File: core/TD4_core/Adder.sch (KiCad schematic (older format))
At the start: 30 parts

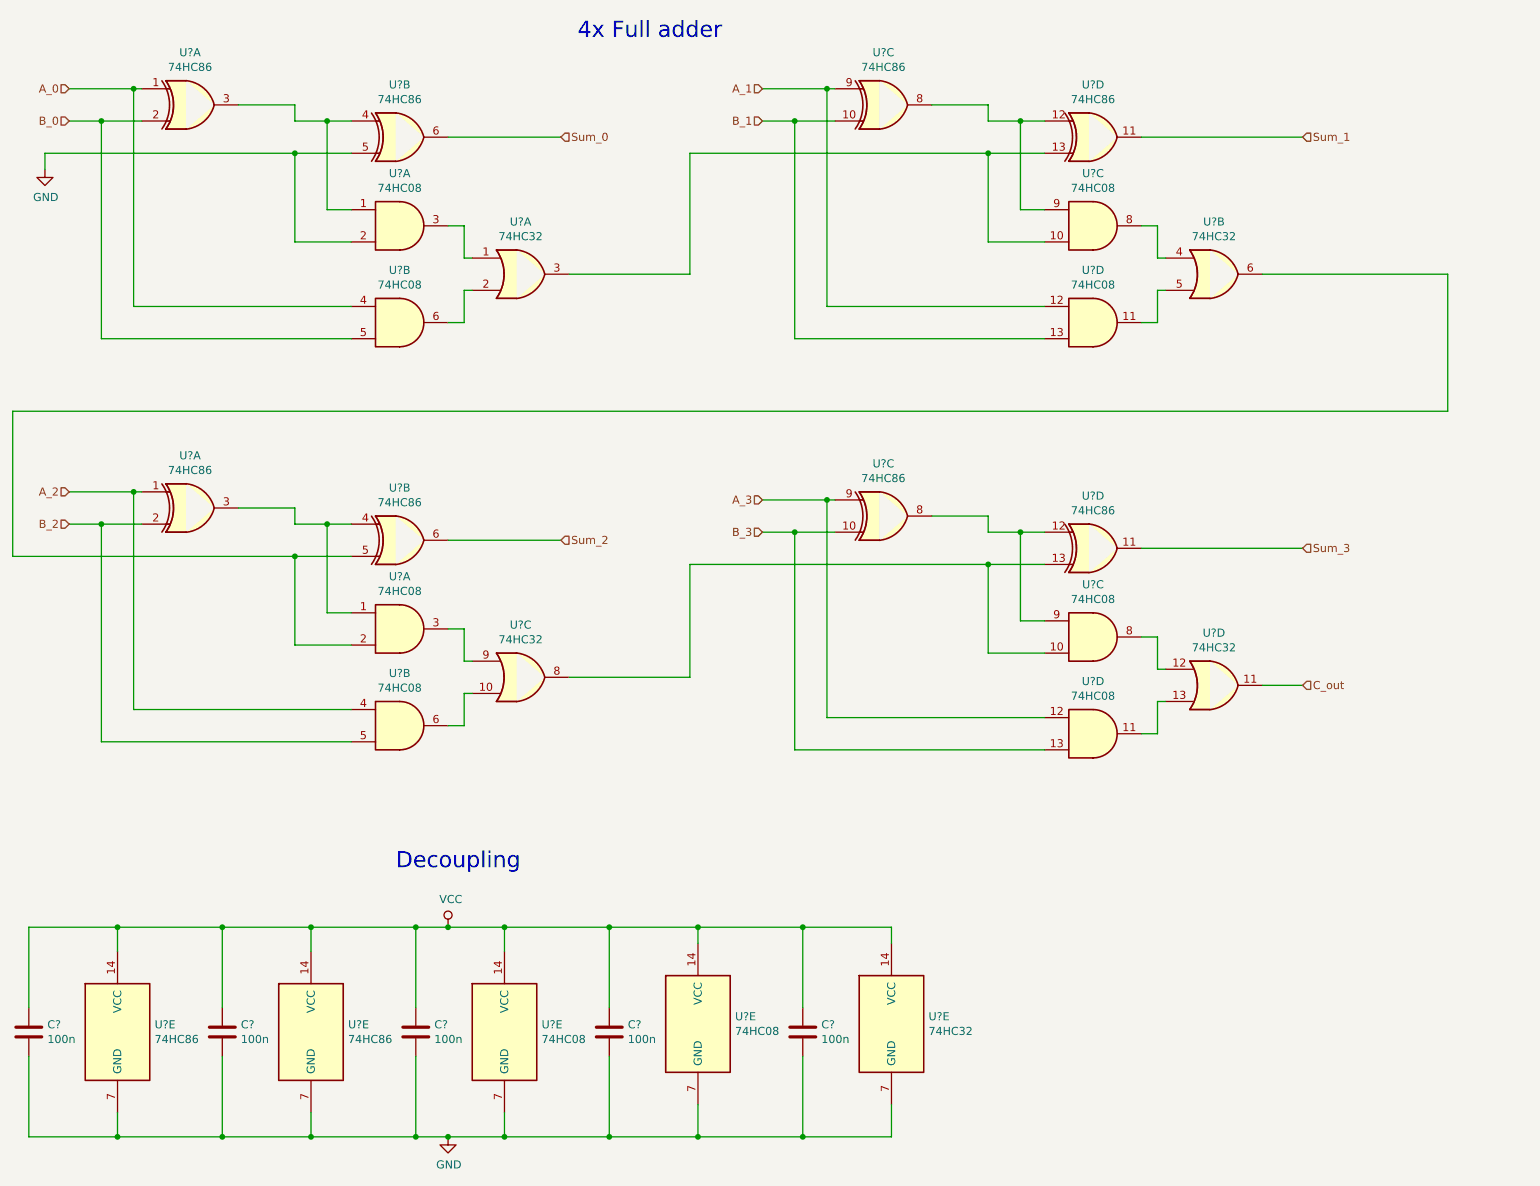
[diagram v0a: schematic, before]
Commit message: RAM refactoring goes on
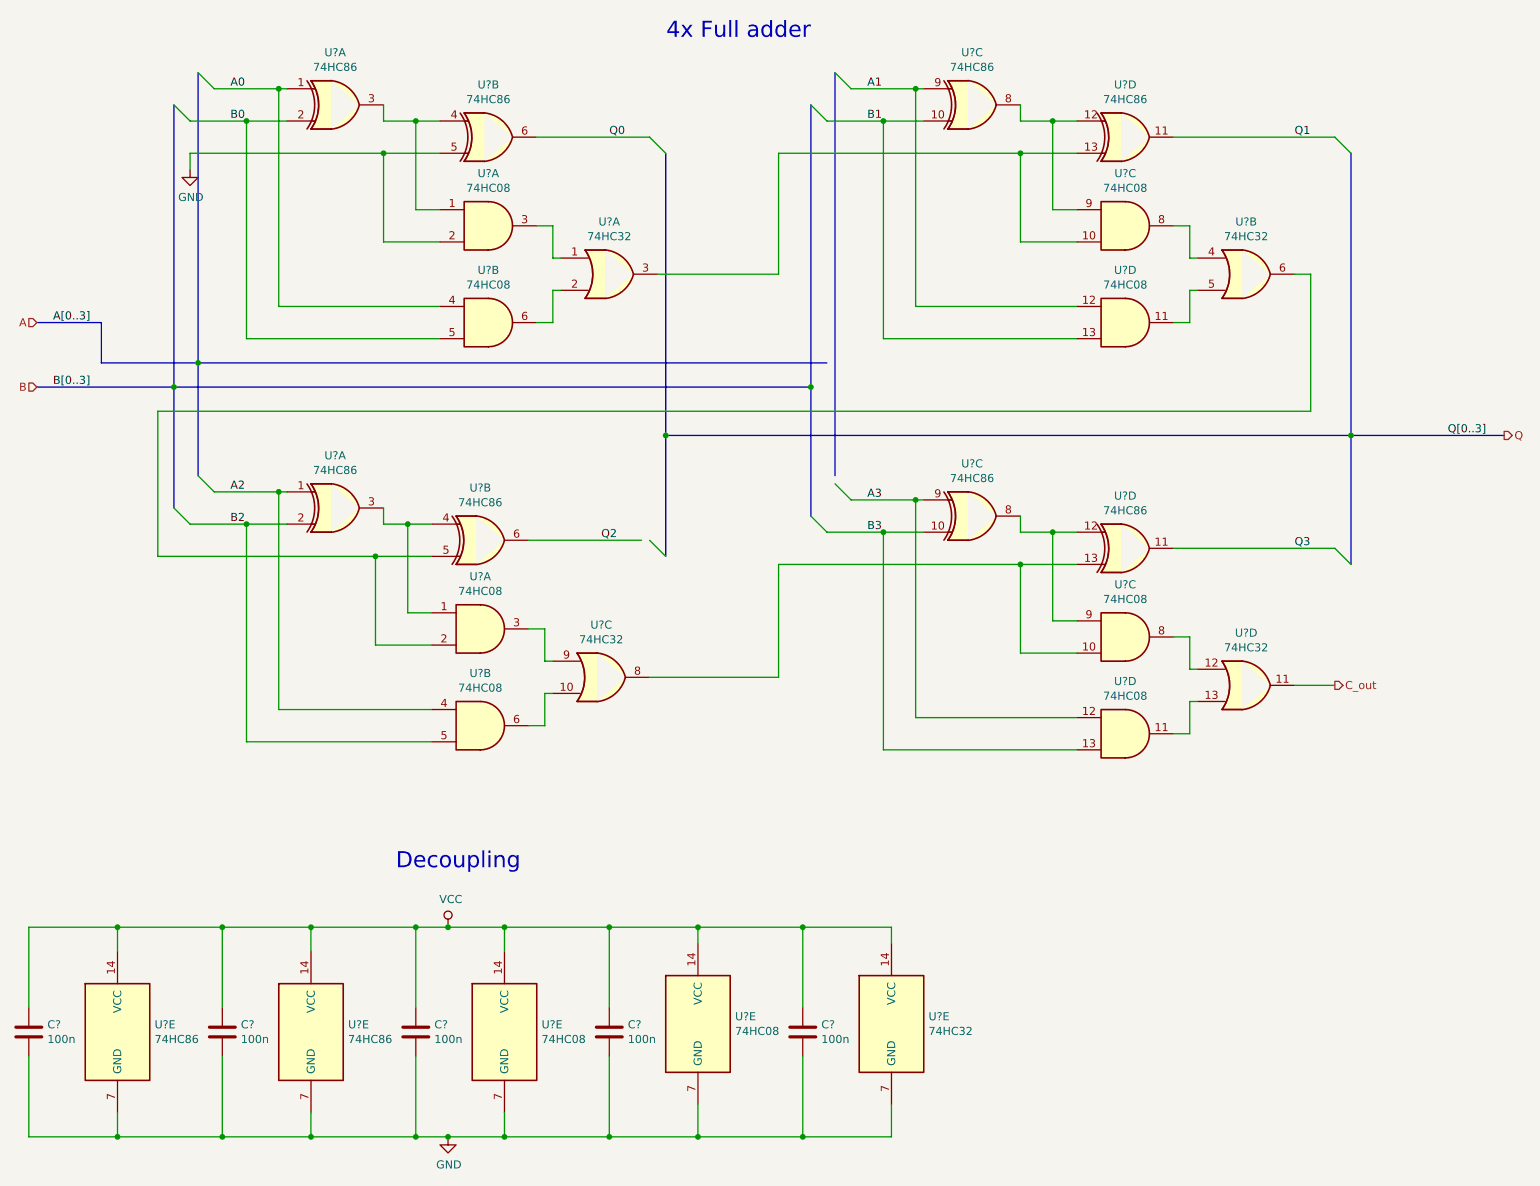
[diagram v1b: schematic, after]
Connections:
- net A_0 renamed A0
- net A_1 renamed A1
- net A_2 renamed A2
- net A_3 renamed A3
- net B_0 renamed B0
- net B_1 renamed B1
- net B_2 renamed B2
- net B_3 renamed B3
- net Sum_0 renamed Q0
- net Sum_1 renamed Q1
- net Sum_2 renamed Q2
- net Sum_3 renamed Q3
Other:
- moved on the sheet: U?A, U?B, U?C, U?D
